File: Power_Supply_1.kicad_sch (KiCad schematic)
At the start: 14 parts

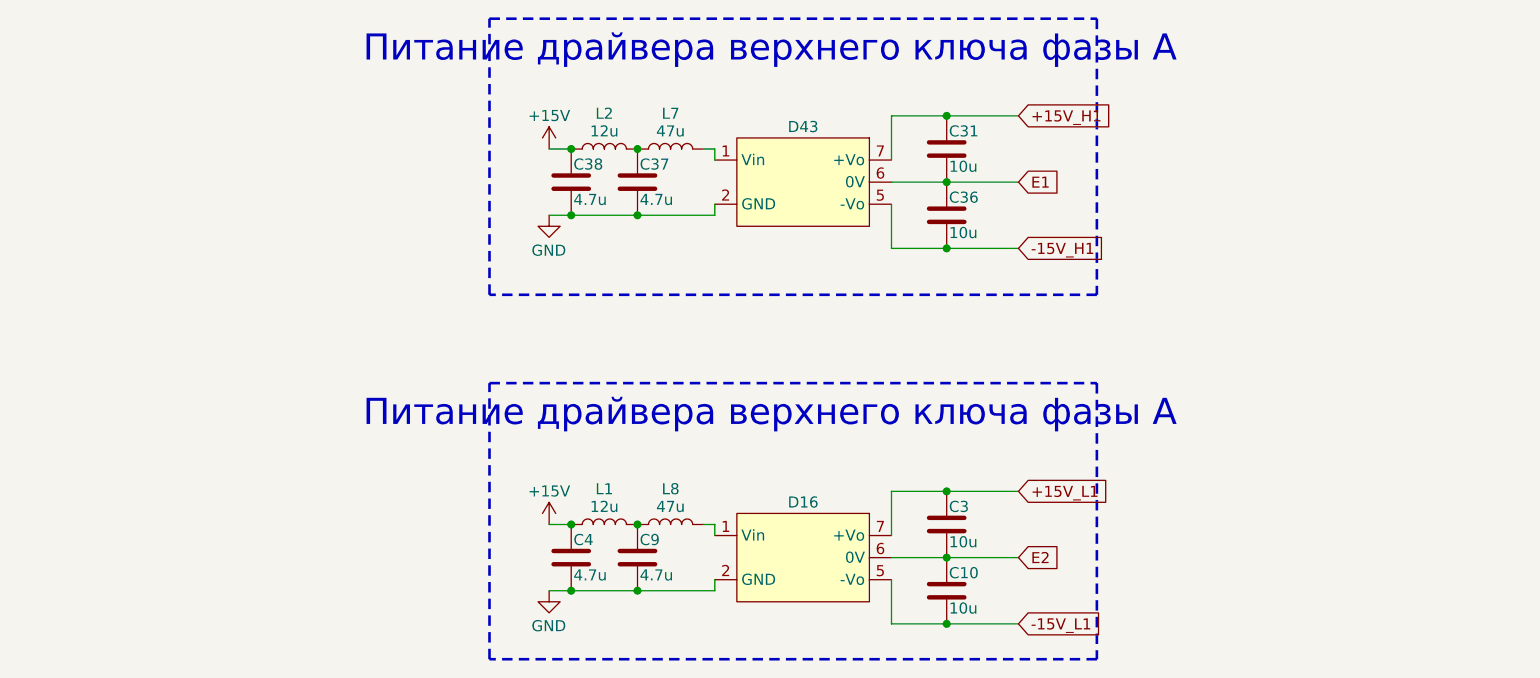
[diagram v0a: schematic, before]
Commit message: VER2.2.1: создал папку для производственных доков
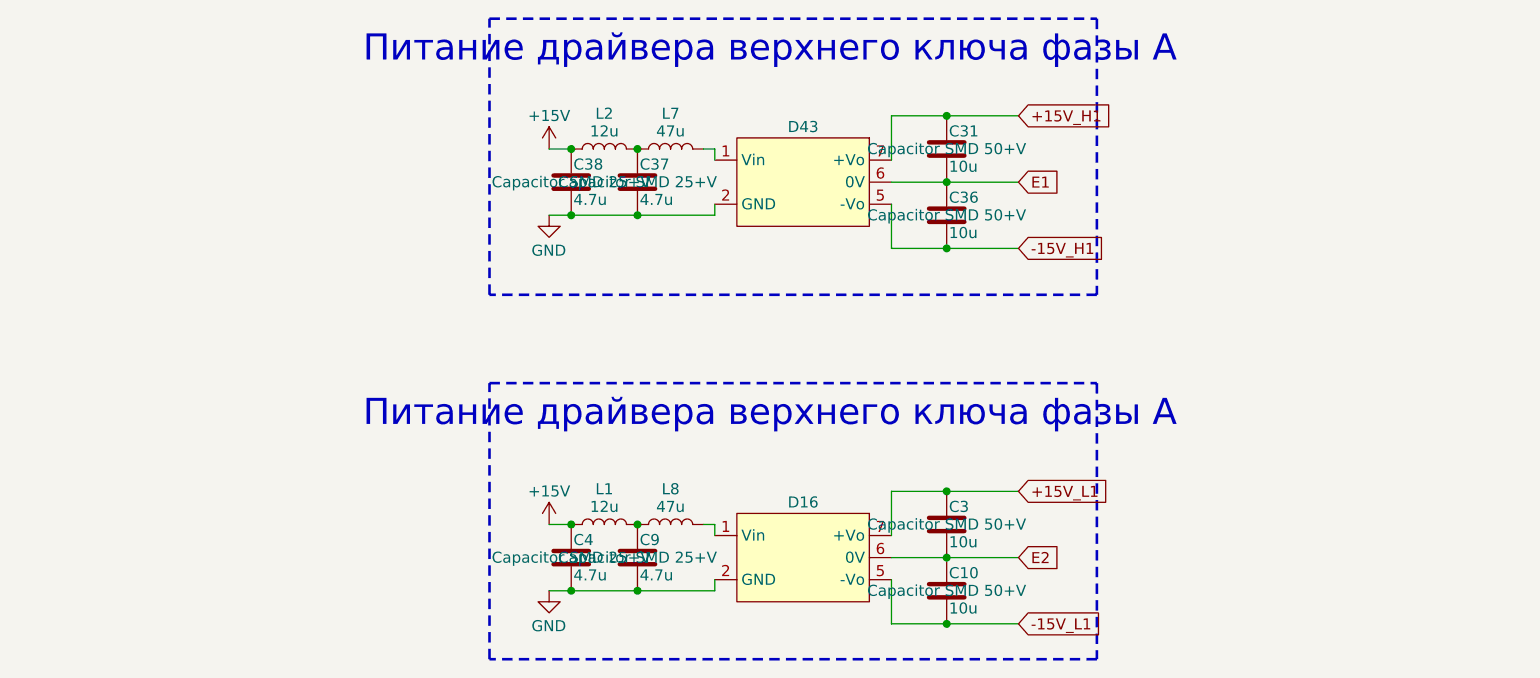
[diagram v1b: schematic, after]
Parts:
- C10, C3, C31, C36: Description P/N (none) -> Capacitor SMD 50+V
- C37, C38, C4, C9: Description P/N (none) -> Capacitor SMD 25+V
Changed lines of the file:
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@@
 			)
 		)
-		(property "Description P/N" ""
+		(property "Description P/N" "Capacitor SMD 50+V"
 			(at 171.45 127 0)
 			(effects
@@
 			)
 		)
-		(property "Description P/N" ""
+		(property "Description P/N" "Capacitor SMD 50+V"
 			(at 171.45 91.44 0)
 			(effects
@@
 			)
 		)
-		(property "Description P/N" ""
+		(property "Description P/N" "Capacitor SMD 25+V"
 			(at 135.89 87.63 0)
 			(effects
@@
 			)
 		)
-		(property "Description P/N" ""
+		(property "Description P/N" "Capacitor SMD 25+V"
 			(at 128.27 130.81 0)
 			(effects
@@
 			)
 		)
-		(property "Description P/N" ""
+		(property "Description P/N" "Capacitor SMD 25+V"
 			(at 128.27 87.63 0)
 			(effects
@@
 			)
 		)
-		(property "Description P/N" ""
+		(property "Description P/N" "Capacitor SMD 25+V"
 			(at 135.89 130.81 0)
 			(effects
@@
 			)
 		)
-		(property "Description P/N" ""
+		(property "Description P/N" "Capacitor SMD 50+V"
 			(at 171.45 83.82 0)
 			(effects
@@
 			)
 		)
-		(property "Description P/N" ""
+		(property "Description P/N" "Capacitor SMD 50+V"
 			(at 171.45 134.62 0)
 			(effects

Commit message: VER2.2.1: исправил все доки
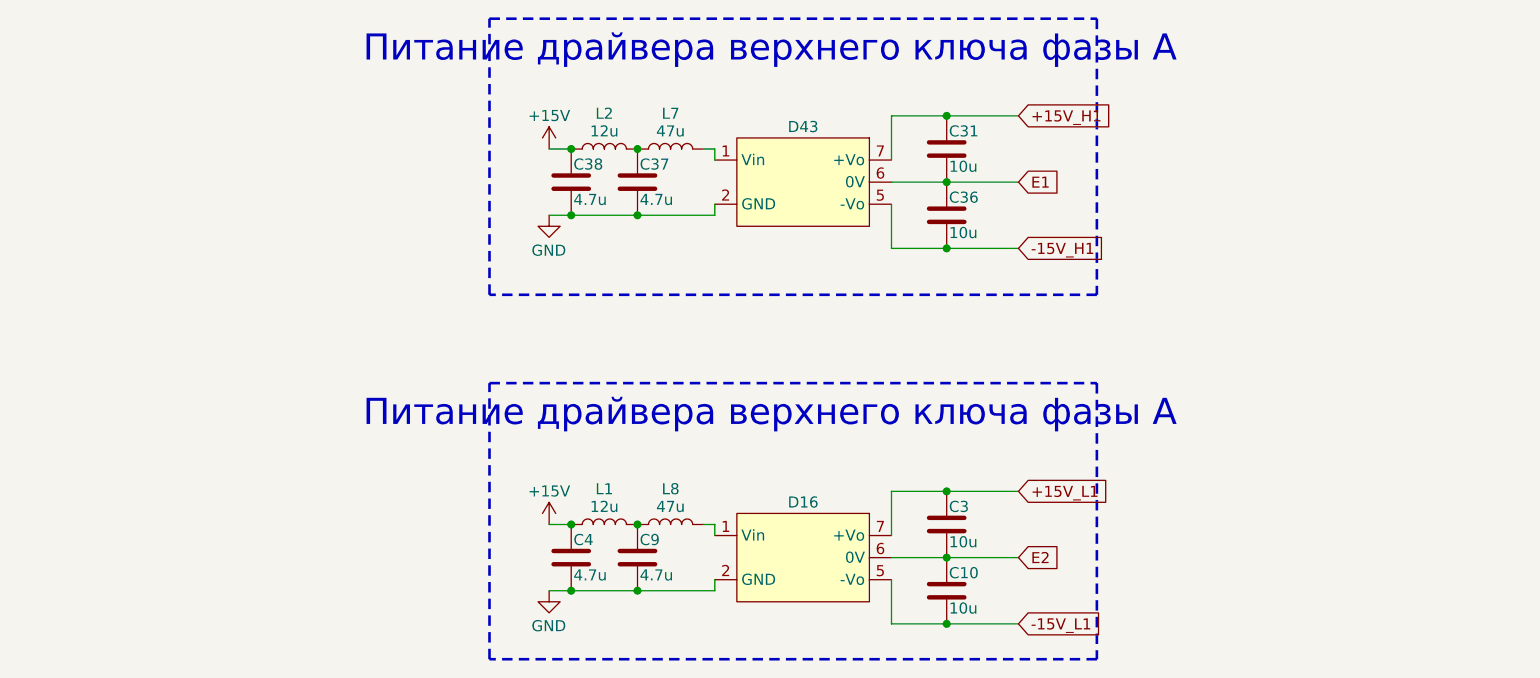
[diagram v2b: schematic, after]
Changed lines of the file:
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@@
 		(date "2025-06-04")
 		(company "ООО \"ЭТТ\"")
+		(comment 1 "НВЦТ.EVP150-2-1.2000.120_v1 Э3")
 	)
 	(rectangle
@@
 					(size 1.27 1.27)
 				)
+				(hide yes)
 			)
 		)
@@
 					(size 1.27 1.27)
 				)
+				(hide yes)
 			)
 		)
@@
 					(size 1.27 1.27)
 				)
+				(hide yes)
 			)
 		)
@@
 					(size 1.27 1.27)
 				)
+				(hide yes)
 			)
 		)
@@
 					(size 1.27 1.27)
 				)
+				(hide yes)
 			)
 		)
@@
 					(size 1.27 1.27)
 				)
+				(hide yes)
 			)
 		)
@@
 					(size 1.27 1.27)
 				)
+				(hide yes)
 			)
 		)
@@
 					(size 1.27 1.27)
 				)
-			)
-		)
+				(hide yes)
+			)
+		)
